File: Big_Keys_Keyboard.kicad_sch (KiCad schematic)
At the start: 13 parts, among them J1 SM04B-SRSS-TB(LF)(SN), J2 SM04B-SRSS-TB(LF)(SN), U1 MX1A-11NN, U2 MX1A-11NN, U3 MX1A-11NN, U4 MX1A-11NN

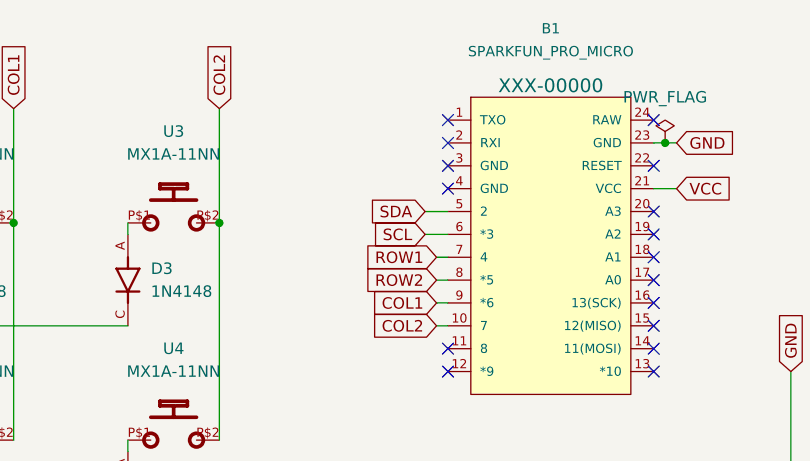
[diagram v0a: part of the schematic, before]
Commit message: printable design ready
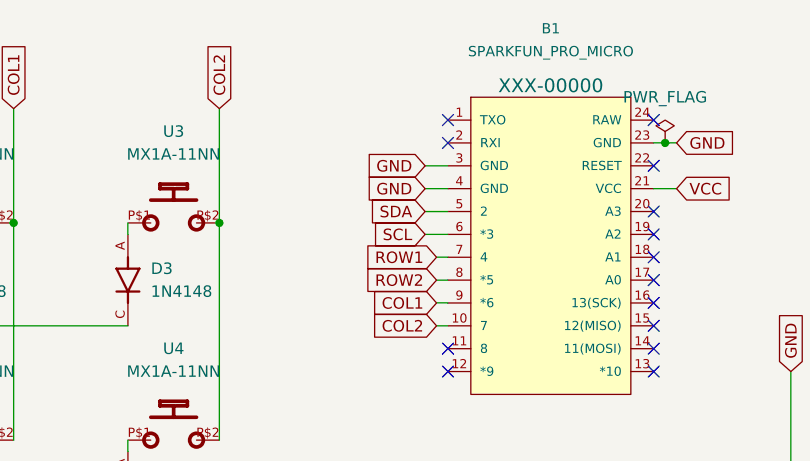
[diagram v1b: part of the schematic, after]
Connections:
- net GND: now also B1.3 (GND), B1.4 (GND)
- no-connect marks 16 -> 14
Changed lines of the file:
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@@
   (no_connect (at 193.04 92.71))
   (no_connect (at 193.04 107.95))
-  (no_connect (at 170.18 87.63))
   (no_connect (at 193.04 102.87))
   (no_connect (at 170.18 82.55))
   (no_connect (at 170.18 85.09))
   (no_connect (at 193.04 100.33))
-  (no_connect (at 170.18 90.17))
   (no_connect (at 193.04 97.79))
   (no_connect (at 193.04 105.41))
@@
     (stroke (width 0) (type default) (color 0 0 0 0))
   )
+  (wire (pts (xy 167.64 87.63) (xy 170.18 87.63))
+    (stroke (width 0) (type default) (color 0 0 0 0))
+  )
   (wire (pts (xy 219.71 139.7) (xy 220.98 139.7))
     (stroke (width 0) (type default) (color 0 0 0 0))
@@
     (stroke (width 0) (type default) (color 0 0 0 0))
   )
+  (wire (pts (xy 167.64 90.17) (xy 170.18 90.17))
+    (stroke (width 0) (type default) (color 0 0 0 0))
+  )
   (wire (pts (xy 220.98 139.7) (xy 224.79 139.7))
     (stroke (width 0) (type default) (color 0 0 0 0))
@@
     )
   )
+  (global_label "GND" (shape input) (at 167.64 87.63 180) (fields_autoplaced)
+    (effects (font (size 1.27 1.27)) (justify right))
+    (property "Intersheet References" "${INTERSHEET_REFS}" (id 0) (at 161.3564 87.5506 0)
+      (effects (font (size 1.27 1.27)) (justify right) hide)
+    )
+  )
   (global_label "GND" (shape input) (at 219.71 142.24 180) (fields_autoplaced)
     (effects (font (size 1.27 1.27)) (justify right))
@@
       (effects (font (size 1.27 1.27)) (justify right) hide)
     )
+  )
+  (global_label "GND" (shape input) (at 167.64 90.17 180) (fields_autoplaced)
+    (effects (font (size 1.27 1.27)) (justify right))
+    (property "Intersheet References" "${INTERSHEET_REFS}" (id 0) (at 161.3564 90.0906 0)
+      (effects (font (size 1.27 1.27)) (justify right) hide)
+    )
